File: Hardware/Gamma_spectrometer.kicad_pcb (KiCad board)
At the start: 2 copper layers, 76.1 x 31 mm, 47 parts, among them J1 Conn_01x04, J10 Test Pad, J11 Test Pad, J12 Test Pad, J2 Conn_01x04, J3 Conn_01x01, J4 Conn_01x04, J5 Test Pad, J6 Test Pad, J7 Test Pad, J8 Test Pad, J9 Test Pad, Q1 2N7002, U11 ATtiny1616-M, U2 LM317L_SO8, U3 OPA356xxDBV, U4 OPA357AIDVBR, U5 OPA357AIDVBR, U6 LMV7219M7, U7 OPA356xxDBV, U8 FODM217A

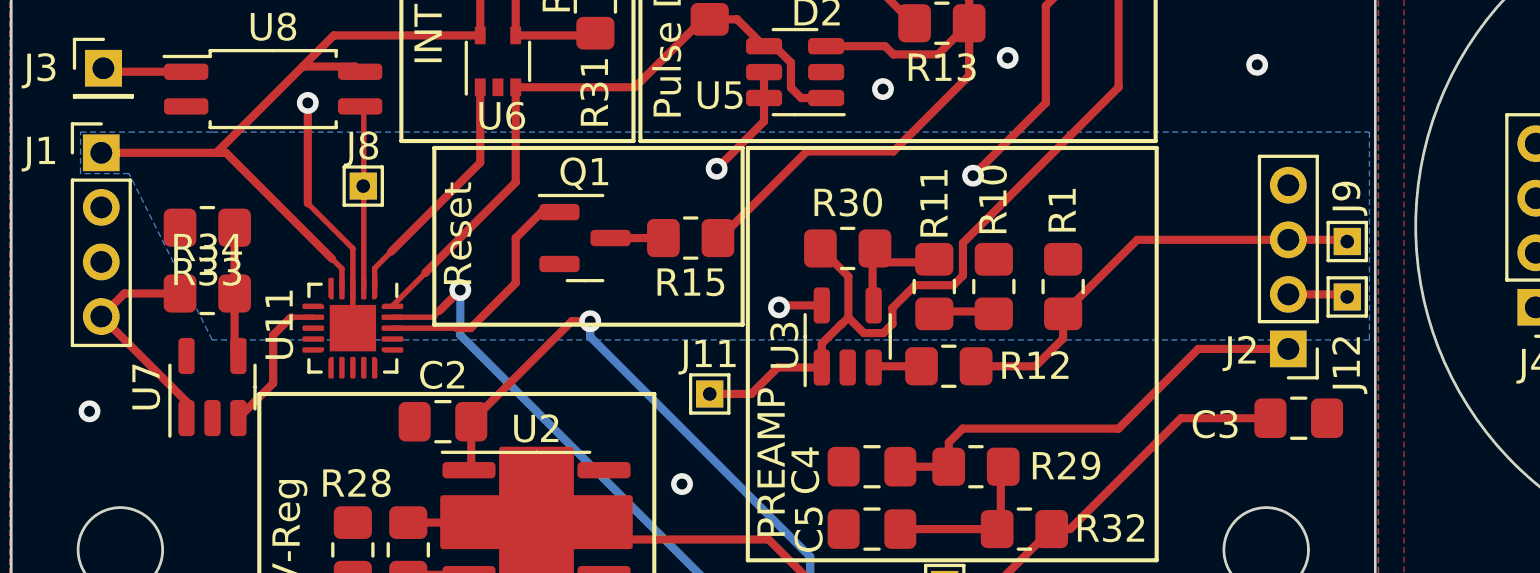
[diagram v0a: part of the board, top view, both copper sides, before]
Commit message: stuff
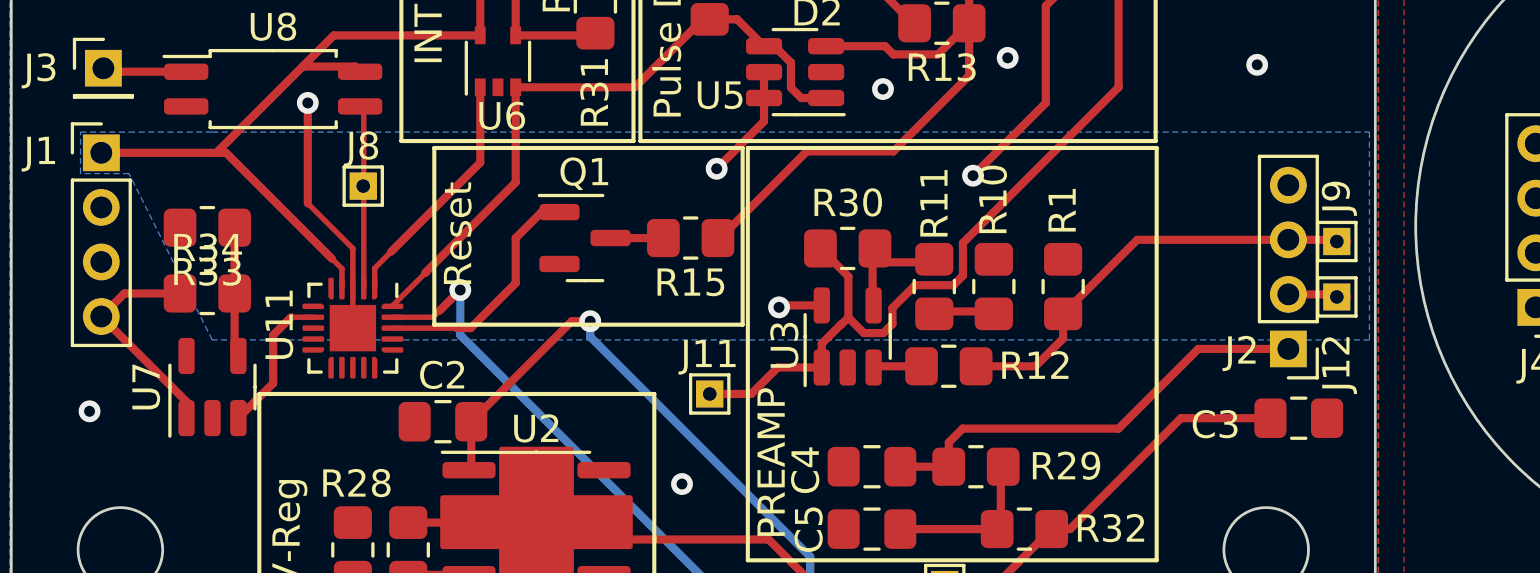
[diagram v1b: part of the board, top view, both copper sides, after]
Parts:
- moved J12 0.38 mm to (148.6, 117.7)
- moved J9 0.38 mm to (148.6, 115.7)
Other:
- board text added: "Alignment"
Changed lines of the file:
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@@
       (sketchpadsonfab false)
       (subtractmaskfromsilk false)
-      (outputformat 1)
+      (outputformat 4)
       (mirror false)
       (drillshape 0)
       (scaleselection 1)
-      (outputdirectory "")
+      (outputdirectory "Pcb file/")
     )
   )
@@
     (fp_line (start -1 0.625) (end -1 -0.625) (layer "F.Fab") (width 0.1))
     (fp_line (start -1 -0.625) (end 1 -0.625) (layer "F.Fab") (width 0.1))
-    (pad "1" smd roundrect (at -1 0 180) (size 1.2 1.4) (layers "F.Cu" "F.Paste" "F.Mask") (roundrect_rratio 0.208333)
+    (pad "1" smd roundrect (at -1 0 180) (size 1.2 1.4) (layers "F.Cu" "F.Paste" "F.Mask") (roundrect_rratio 0.2083333333)
       (net 42 "Net-(R33-Pad1)") (pintype "passive"))
-    (pad "2" smd roundrect (at 1 0 180) (size 1.2 1.4) (layers "F.Cu" "F.Paste" "F.Mask") (roundrect_rratio 0.208333)
+    (pad "2" smd roundrect (at 1 0 180) (size 1.2 1.4) (layers "F.Cu" "F.Paste" "F.Mask") (roundrect_rratio 0.2083333333)
       (net 2 "GND") (pintype "passive"))
     (model "${KICAD6_3DMODEL_DIR}/Resistor_SMD.3dshapes/R_0805_2012Metric.wrl"
@@
     (fp_line (start 1 0.625) (end -1 0.625) (layer "F.Fab") (width 0.1))
     (fp_line (start 1 -0.625) (end 1 0.625) (layer "F.Fab") (width 0.1))
-    (pad "1" smd roundrect (at -1 0) (size 1.2 1.4) (layers "F.Cu" "F.Paste" "F.Mask") (roundrect_rratio 0.208333)
+    (pad "1" smd roundrect (at -1 0) (size 1.2 1.4) (layers "F.Cu" "F.Paste" "F.Mask") (roundrect_rratio 0.2083333333)
       (net 34 "OutSignal") (pintype "passive"))
-    (pad "2" smd roundrect (at 1 0) (size 1.2 1.4) (layers "F.Cu" "F.Paste" "F.Mask") (roundrect_rratio 0.208333)
+    (pad "2" smd roundrect (at 1 0) (size 1.2 1.4) (layers "F.Cu" "F.Paste" "F.Mask") (roundrect_rratio 0.2083333333)
       (net 42 "Net-(R33-Pad1)") (pintype "passive"))
     (model "${KICAD6_3DMODEL_DIR}/Resistor_SMD.3dshapes/R_0805_2012Metric.wrl"
@@
   )
   (footprint "TestPoint:TestPoint_THTPad_1.0x1.0mm_Drill0.5mm" (layer "F.Cu")
-    (at 148.971 115.697)
+    (at 148.59 115.697)
     (descr "THT rectangular pad as test Point, square 1.0mm side length, hole diameter 0.5mm")
     (tags "test point THT pad rectangle square")
@@
     (fp_line (start -1 0.625) (end -1 -0.625) (layer "F.Fab") (width 0.1))
     (fp_line (start 1 -0.625) (end 1 0.625) (layer "F.Fab") (width 0.1))
-    (pad "1" smd roundrect (at -1 0 90) (size 1.2 1.4) (layers "F.Cu" "F.Paste" "F.Mask") (roundrect_rratio 0.208333)
+    (pad "1" smd roundrect (at -1 0 90) (size 1.2 1.4) (layers "F.Cu" "F.Paste" "F.Mask") (roundrect_rratio 0.2083333333)
       (net 8 "SIPM") (pintype "passive"))
-    (pad "2" smd roundrect (at 1 0 90) (size 1.2 1.4) (layers "F.Cu" "F.Paste" "F.Mask") (roundrect_rratio 0.208333)
+    (pad "2" smd roundrect (at 1 0 90) (size 1.2 1.4) (layers "F.Cu" "F.Paste" "F.Mask") (roundrect_rratio 0.2083333333)
       (net 2 "GND") (pintype "passive"))
     (model "${KICAD6_3DMODEL_DIR}/Resistor_SMD.3dshapes/R_0805_2012Metric.wrl"
@@
   )
   (footprint "TestPoint:TestPoint_THTPad_1.0x1.0mm_Drill0.5mm" (layer "F.Cu")
-    (at 148.971 117.729)
+    (at 148.59 117.729)
     (descr "THT rectangular pad as test Point, square 1.0mm side length, hole diameter 0.5mm")
     (tags "test point THT pad rectangle square")
@@
   (gr_circle locked (center 146 104) (end 147.55 104) (layer "Edge.Cuts") (width 0.1) (fill none))
   (gr_circle locked (center 104 127) (end 105.55 127) (layer "Edge.Cuts") (width 0.1) (fill none))
+  (gr_rect (start 94.742 92.71) (end 177.927 136.017) (layer "User.1") (width 0.15) (fill none))
   (gr_text "INT GEN" (at 115.316 106.426 90) (layer "F.SilkS")
     (effects (font (size 1 1) (thickness 0.15)))
@@
     (effects (font (size 1 1) (thickness 0.15)))
   )
+  (gr_text "Alignment" (at 103.886 96.139) (layer "User.1")
+    (effects (font (size 1 1) (thickness 0.15)))
+  )
+  (target plus (at 151.13 132.969) (size 5) (width 0.1) (layer "Edge.Cuts"))
+  (target plus (at 98.425 132.715) (size 5) (width 0.1) (layer "Edge.Cuts"))
+  (target plus (at 98.679 98.679) (size 5) (width 0.1) (layer "Edge.Cuts"))
+  (target plus (at 151.511 98.552) (size 5) (width 0.1) (layer "Edge.Cuts"))
   (segment (start 127.593749 111.293251) (end 127.593749 110.437375) (width 0.3) (layer "F.Cu") (net 1))
   (segment (start 129.71025 118.0395) (end 128.2135 118.0395) (width 0.3) (layer "F.Cu") (net 1))
